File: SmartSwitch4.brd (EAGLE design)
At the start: 40 x 44 mm, 9 parts, among them SW1 SWITCH-SPST-ILLUMINATED, SW2 SWITCH-SPST-ILLUMINATED, SW3 SWITCH-SPST-ILLUMINATED, SW4 SWITCH-SPST-ILLUMINATED

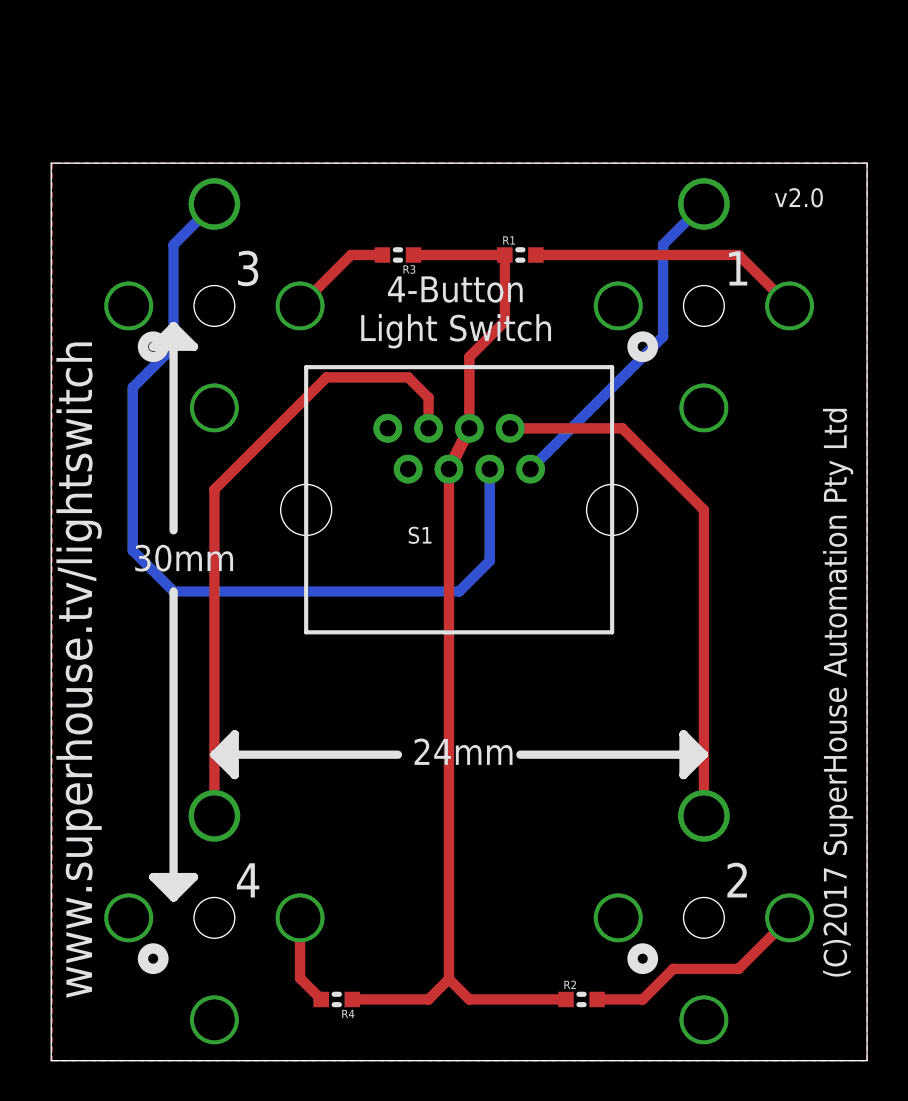
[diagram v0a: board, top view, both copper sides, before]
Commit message: Routing
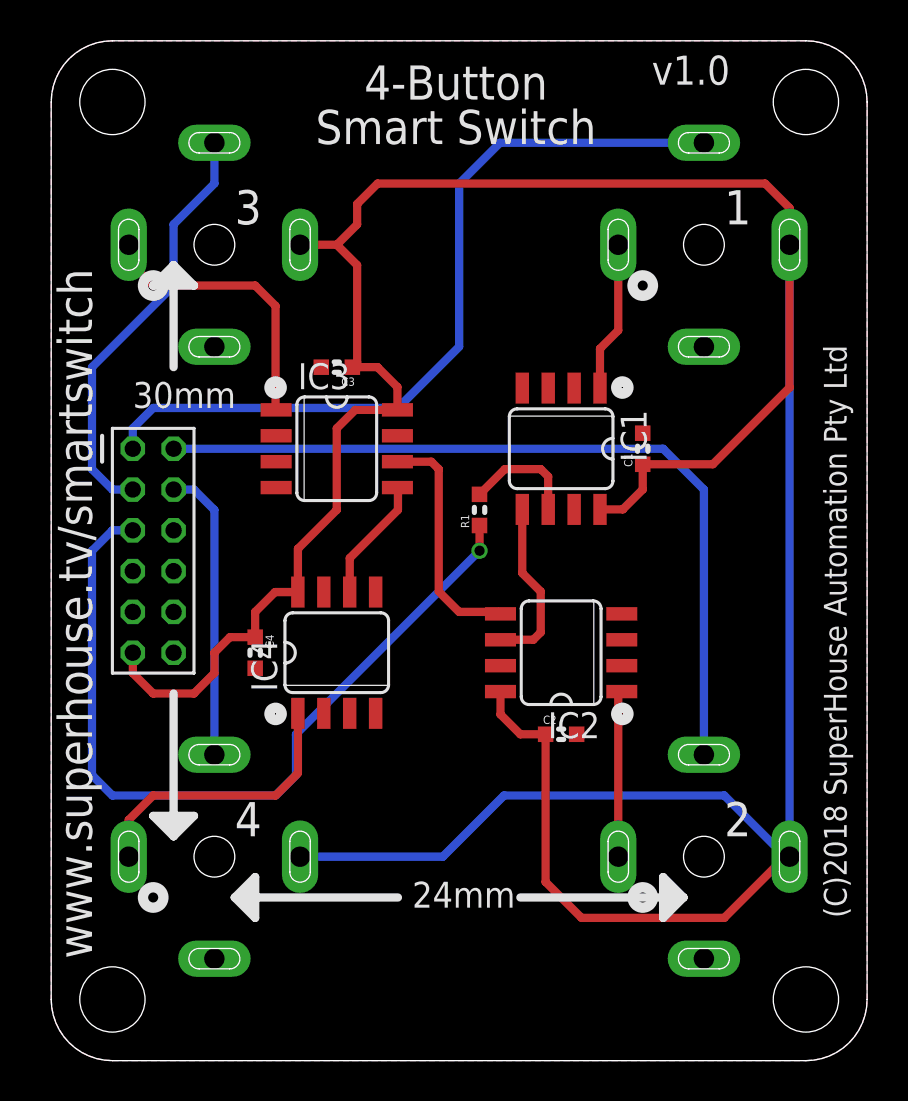
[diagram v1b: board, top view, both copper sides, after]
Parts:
- removed R2, R3, R4: 3K3, freetronics-jon:0603
- removed S1: RJ45, freetronics-jon:RJ45
- added C1, C2, C3, C4: 1uF, freetronics-jon:0603
- added H1: M06X22MM, freetronics-jon:2X6-2MM
- added IC1, IC2, IC3, IC4: WS2811-SOP8, freetronics-jon:SO08-SKINNYPADS
- R1: value 3K3 -> 100R
- moved R1 12.7 mm to (21.0, 27.0), turned to 90 degrees
- moved SW1 3.00 mm to (32.0, 40.0)
- moved SW2 3.00 mm to (32.0, 10.0)
- moved SW3 3.00 mm to (8.00, 40.0)
- moved SW4 3.00 mm to (8.00, 10.0)
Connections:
- removed net +12V: R1.1, R2.1, R3.1, R4.1, S1.4, S1.5
- removed net N$2: S1.3, SW3.3
- removed net N$3: S1.6, SW4.3
- removed net N$4: S1.1, SW1.3
- removed net N$5: S1.2, SW2.3
- removed net N$7: R3.2, SW3.2
- removed net N$8: R4.2, SW4.2
- new net 5V: C1.1, C2.1, C3.1, C4.1, H1.11, IC1.8, IC2.8, IC3.8, IC4.8, SW1.2, SW2.2, SW3.2, SW4.2
- new net DATA_1: H1.1, SW1.3
- new net DATA_2: H1.2, SW2.3
- new net DATA_3: H1.3, SW3.3
- new net DATA_4: H1.4, SW4.3
- new net DATA_5: H1.5, R1.1
- new net DATA_6: H1.6
- new net DATA_7: H1.7
- new net DATA_8: H1.8
- new net LED1_K: IC1.1, SW1.1
- new net LED2_K: IC2.1, SW2.1
- new net LED3_K: IC3.1, SW3.1
- new net LED4_K: IC4.1, SW4.1
- new net N$12: IC2.5, IC3.6
- new net N$13: IC3.5, IC4.6
- new net RESET: H1.12
- new net VIN: H1.9
- net GND: now also C1.2, C2.2, C3.2, C4.2, H1.10, IC1.4, IC2.4, IC3.4, IC4.4; no longer S1.7, S1.8, SW1.1, SW2.1, SW3.1, SW4.1
- net N$1: now also IC1.6, R1.2; no longer R2.2, SW2.2
- net N$6: now also IC1.5, IC2.6; no longer R1.2, SW1.2
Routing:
- net 5V: track 0.00 -> 164.3 mm
- net +12V: track 52.2 -> 0.00 mm
- net N$2: track 42.1 -> 0.00 mm
- net DATA_5: track 0.00 -> 40.2 mm, vias 0 -> 1
- net DATA_2: track 0.00 -> 39.8 mm
- net DATA_1: track 0.00 -> 39.5 mm
- net N$3: track 30.7 -> 0.00 mm
- net N$5: track 26.2 -> 0.00 mm
- net DATA_3: track 0.00 -> 20.9 mm
- net N$4: track 16.5 -> 0.00 mm
- net DATA_4: track 0.00 -> 14.4 mm
- net LED3_K: track 0.00 -> 14.0 mm
- net LED4_K: track 0.00 -> 14.0 mm
- net N$12: track 0.00 -> 11.7 mm
- net LED2_K: track 0.00 -> 8.17 mm
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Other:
- board size 40 x 44 mm -> 40 x 50 mm
- board text added: "(C)2018 SuperHouse Automation Pty Ltd"
- board text added: "4-Button Smart Switch"
- board text added: "v1.0"
- board text added: "www.superhouse.tv/smartswitch"
- board text removed: "(C)2017 SuperHouse Automation Pty Ltd"
- board text removed: "4-Button Light Switch"
- board text removed: "v2.0"
- board text removed: "www.superhouse.tv/lightswitch"
